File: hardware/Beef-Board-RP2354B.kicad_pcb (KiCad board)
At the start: 2 copper layers, 84 x 59.2 mm, 81 parts, among them J1 USB-C DEVICE, J10 VAUX OUT, J11 B1 LEGACY, J12 B2 LEGACY, J13 B3 LEGACY, J14 B4 LEGACY, J15 B5 LEGACY, J16 B6 LEGACY, J17 B7 LEGACY, J18 B8 LEGACY, J19 B9 LEGACY, J2 POWER SELECT, J20 B10 LEGACY, J21 B11 LEGACY, J22 USB COMMON, J3 VAUX 5V INPUT, J31 ENCODER 1, J32 ENCODER 2, J33 AE1 0-5V, J34 AE2 0-5V, J4 USB-C AUX POWER, J40 TT RGB, J41 CENTER BAR RGB, J42 UART A 3V3, J43 UART B 3V3, J5 ENC1 A, J6 ENC1 B, J60 BOOTSEL HEADER, J61 RESET HEADER, J7 ENC2 A, J8 ENC2 B, J9 VAUX OUT, Q1 2N7002, Q10 2N7002, Q11 2N7002, Q2 2N7002, Q3 2N7002, Q4 2N7002, Q5 2N7002, Q6 2N7002, Q7 2N7002, Q8 2N7002, Q9 2N7002, U1 RP2354B, U2 USBLC6-2SC6, U3 AP2112K-3.3, Y1 12MHz CL=10pF

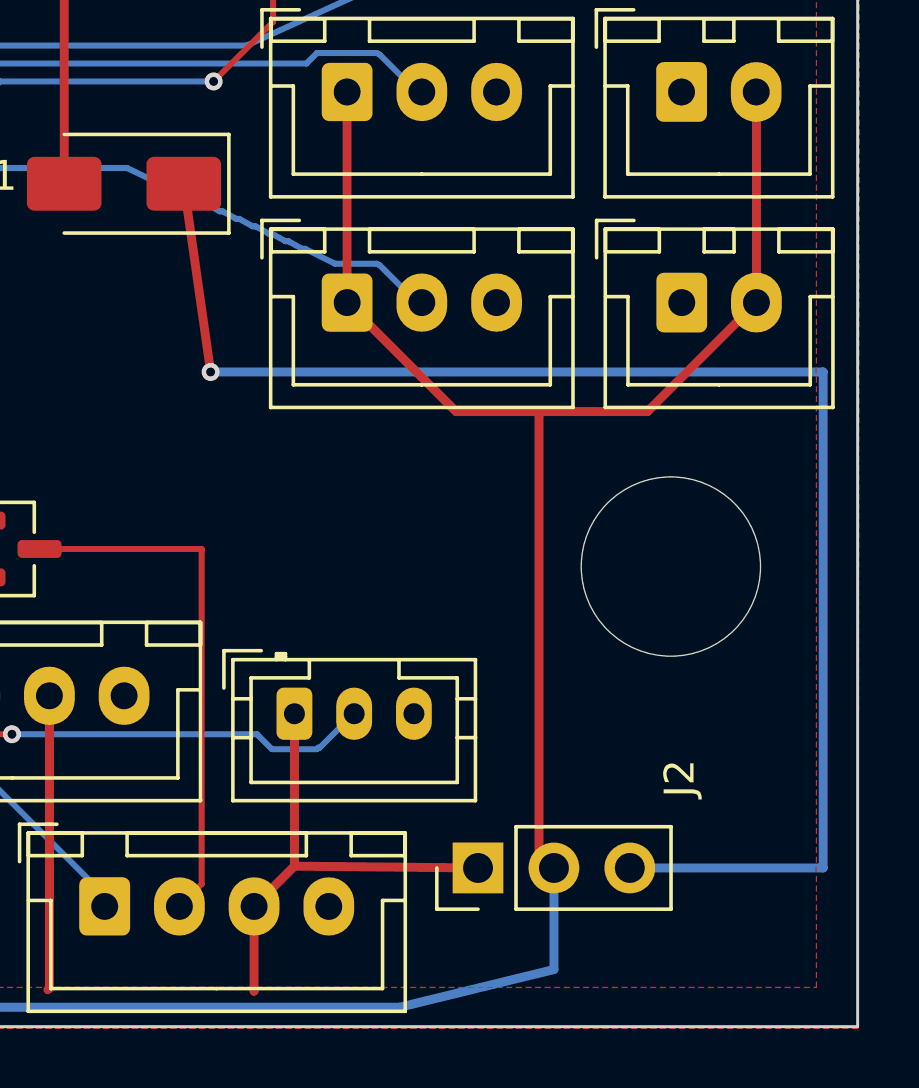
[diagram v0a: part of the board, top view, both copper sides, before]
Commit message: Revert "Replace power switch with selectable header"
This reverts commit b092bcadf7da63c17735a3d5c7bcba7038b5f74d.
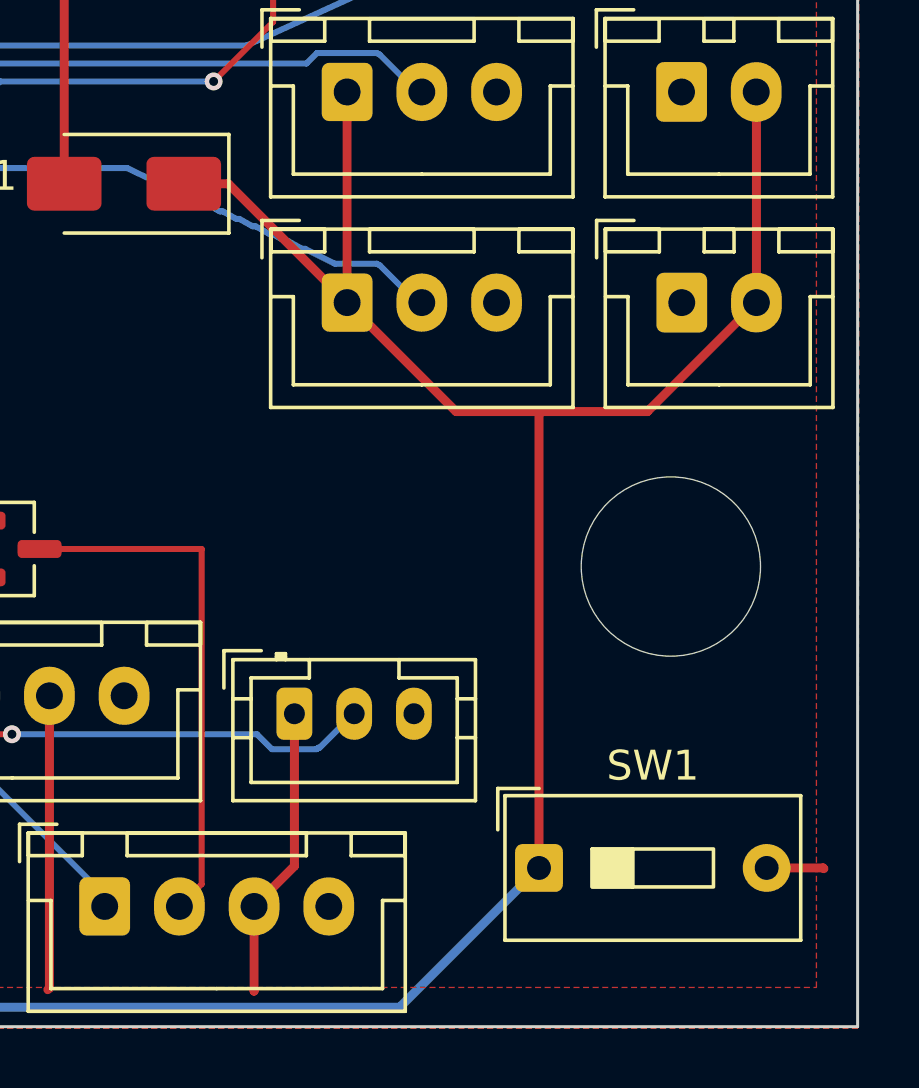
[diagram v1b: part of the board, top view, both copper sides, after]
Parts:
- removed J2: POWER SELECT, PinHeader_1x03_P2.54mm_Vertical
- added SW1: POWER SELECT, Button_Switch_THT:SW_DIP_SPSTx01_Slide_9.78x4.72mm_W7.62mm_P2.54mm, F.Cu at (155.8, 105.9)
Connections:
- D1 pad 1: J4_SEL_5V -> /VAUX_5V
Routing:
- net J4_SEL_5V: track 49.9 -> 0.00 mm, vias 1 -> 0
- net /VAUX_5V: track 137.7 -> 142.2 mm
- net /VBUS_5V: track 153.9 -> 149.7 mm
